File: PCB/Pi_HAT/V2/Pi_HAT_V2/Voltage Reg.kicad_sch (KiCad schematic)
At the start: 7 parts, among them J4 Solenoid I2C, J5 XT60PW-M

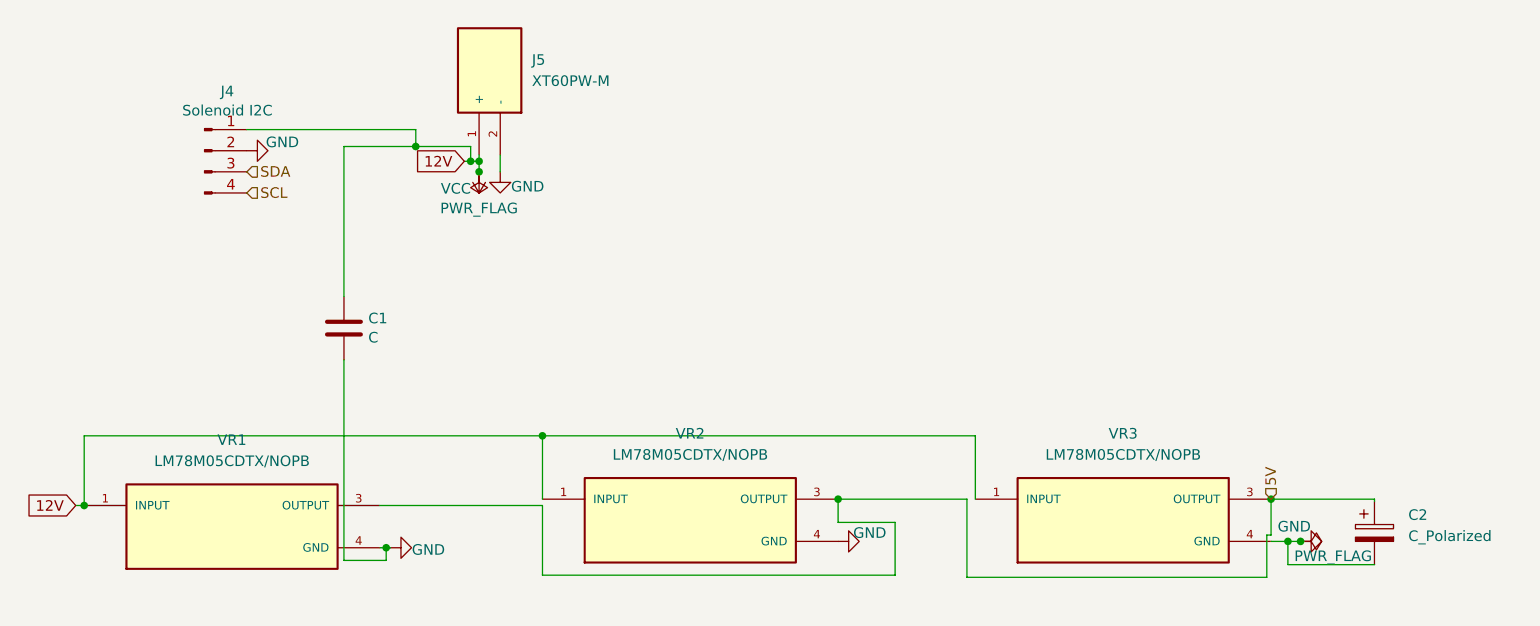
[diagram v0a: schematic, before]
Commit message: Still more to do
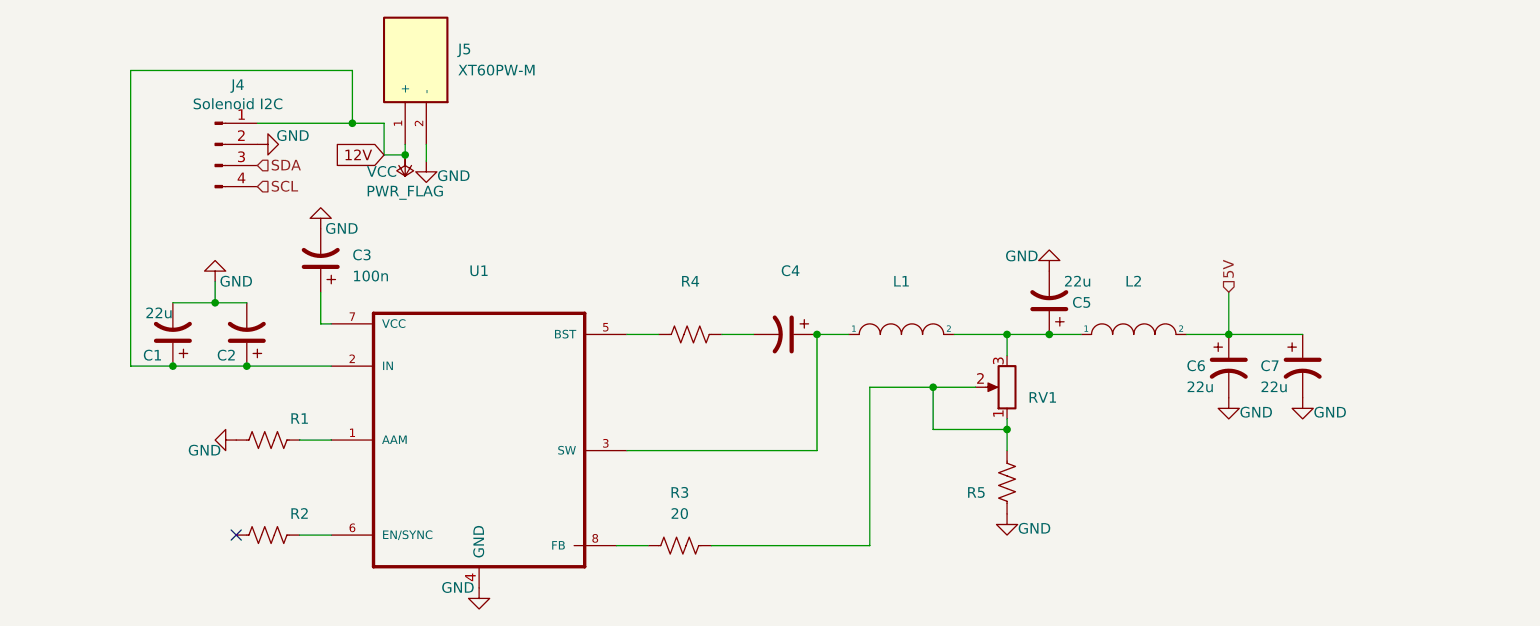
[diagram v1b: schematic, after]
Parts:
- removed C1: C, Capacitor_THT:C_Rect_L7.0mm_W2.5mm_P5.00mm, symbol Device:C
- removed C2: C_Polarized, Capacitor_THT:CP_Radial_D4.0mm_P1.50mm, symbol Device:C_Polarized
- removed VR1, VR2, VR3: LM78M05CDTX/NOPB, .pretty:VREG_L7805ACD2T, symbol LM78M05CDTX_NOPB:LM78M05CDTX/NOPB
- added C1, C5, C6, C7: 22u, symbol Device:C_Polarized_US
- added C2, C4: (no value), symbol Device:C_Polarized_US
- added C3: 100n, symbol Device:C_Polarized_US
- added L1, L2: (no value), symbol pspice:INDUCTOR
- added R1, R2, R4, R5: (no value), symbol Device:R_US
- added R3: 20, symbol Device:R_US
- added RV1: (no value), symbol Device:R_Potentiometer
- added U1: (no value), symbol MP2315GJ-Z:MP2315GJ-Z
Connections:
- net 5V: now also C6.1, C7.1, L2.2
- net GND: now also C1.2, C2.2, C3.2, C5.2, C6.2, C7.2, R1.1, R5.1, U1.4 (GND)
- net VCC: now also C1.1, C2.1, U1.2 (IN)
- new net: R1.2, U1.1 (AAM)
- new net: R4.1, U1.5 (BST)
- new net: C4.2, R4.2
- new net: C4.1, L1.1, U1.3 (SW)
- new net: R2.2, U1.6 (EN/SYNC)
- new net: C3.1, U1.7 (VCC)
- new net: R3.1, U1.8 (FB)
- new net: R3.2, R5.2, RV1.1, RV1.2
- new net: C5.1, L1.2, L2.1, RV1.3
- no-connect marks 0 -> 1
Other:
- moved on the sheet: J4, J5
